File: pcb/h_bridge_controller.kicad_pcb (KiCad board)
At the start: 2 copper layers, 118.1 x 55.1 mm, 48 parts, among them P1 PWR_JACK_2.5x5.5, P2 HEADER_01X03_SMD_RA, P3 HEADER_01X03_SMD_RA, P4 HEADER_01X03_SMD_RA, P5 HEADER_01X03_SMD_RA, P6 HEADER_01X02_SMD_RA, P7 BNC_DOUBLE_RA, SW1 SPST_SLIDE_AS, T1 TERM_BLK_ANG_2_PIN, T2 TERM_BLK_ANG_2_PIN, T3 TERM_BLK_ANG_2_PIN, T4 TERM_BLK_ANG_2_PIN, T5 TERM_BLK_ANG_2_PIN, T6 TERM_BLK_ANG_2_PIN, T7 TERM_BLK_ANG_2_PIN, T8 TERM_BLK_ANG_2_PIN, U1 SSR_DC_6PIN, U2 SSR_DC_6PIN, U3 SSR_DC_6PIN, U4 SSR_DC_6PIN, U5 SSR_DC_6PIN, U6 SSR_DC_6PIN, U7 SSR_DC_6PIN, U8 SSR_DC_6PIN

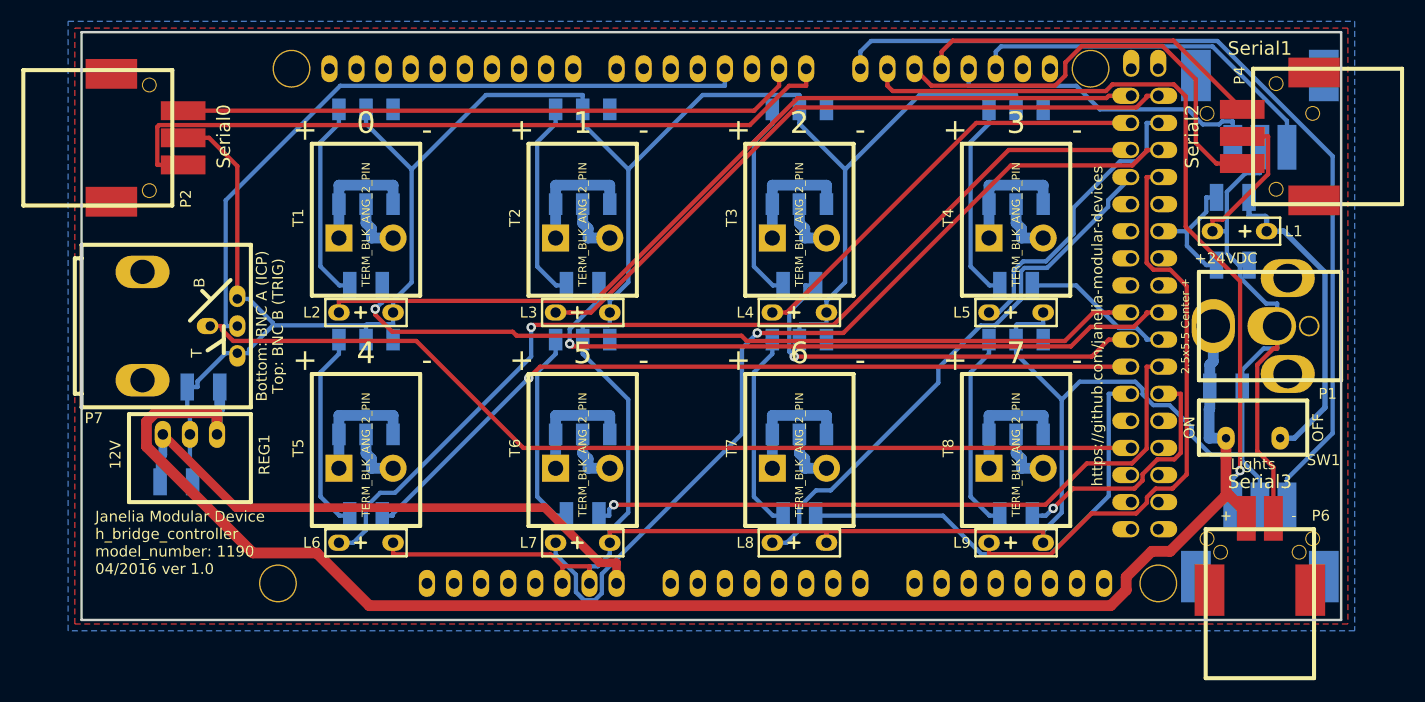
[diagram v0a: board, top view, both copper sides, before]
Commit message: Progress towards pcb1.0.
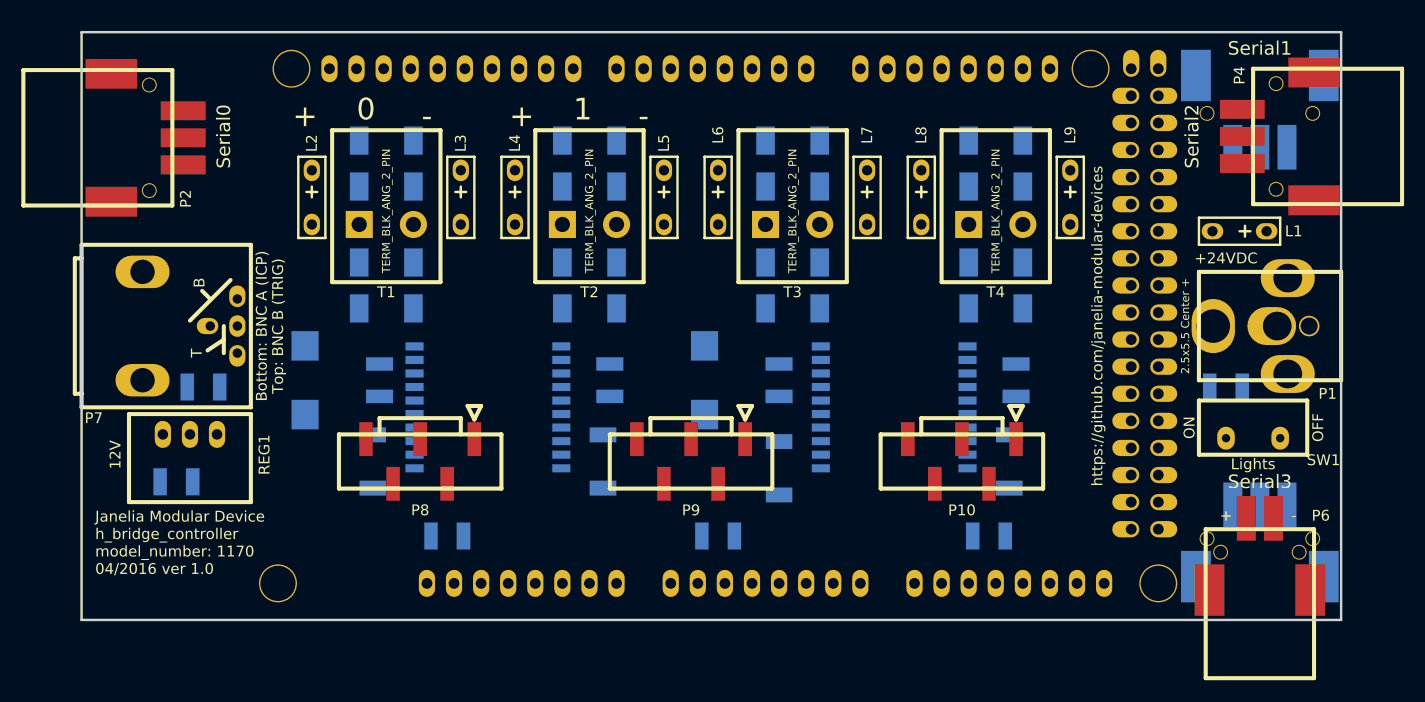
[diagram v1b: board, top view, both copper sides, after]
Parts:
- removed R10, R5, R6: 150, h_bridge_controller:SM1210
- removed T5, T6, T7, T8: TERM_BLK_ANG_2_PIN, h_bridge_controller:TERM_BLK_ANG_2_PIN
- removed U3, U4, U5, U6, U7, U8: SSR_DC_6PIN, h_bridge_controller:ASSR-1611
- added C4: 0.1uF, h_bridge_controller:SM1210, B.Cu at (121.3, 108.0)
- added C5: 0.1uF, h_bridge_controller:SM1210, B.Cu at (142.9, 108.0)
- added C6: 47uF, h_bridge_controller:SM2917_POL, B.Cu at (114.3, 108.0)
- added C7: 0.1uF, h_bridge_controller:SM1210, B.Cu at (158.8, 108.0)
- added C8: 0.1uF, h_bridge_controller:SM1210, B.Cu at (181.0, 108.0)
- added C9: 47uF, h_bridge_controller:SM2917_POL, B.Cu at (151.8, 108.0)
- added D1: diode_schottky_40V_1A, h_bridge_controller:DO-214AC(SMA), B.Cu at (119.4, 87.6)
- added D10: diode_schottky_40V_1A, h_bridge_controller:DO-214AC(SMA), B.Cu at (157.5, 99.1)
- added D11: diode_schottky_40V_1A, h_bridge_controller:DO-214AC(SMA), B.Cu at (162.6, 87.6)
- added D12: diode_schottky_40V_1A, h_bridge_controller:DO-214AC(SMA), B.Cu at (162.6, 99.1)
- added D13: diode_schottky_40V_1A, h_bridge_controller:DO-214AC(SMA), B.Cu at (176.5, 87.6)
- added D14: diode_schottky_40V_1A, h_bridge_controller:DO-214AC(SMA), B.Cu at (176.5, 99.1)
- added D15: diode_schottky_40V_1A, h_bridge_controller:DO-214AC(SMA), B.Cu at (181.6, 87.6)
- added D16: diode_schottky_40V_1A, h_bridge_controller:DO-214AC(SMA), B.Cu at (181.6, 99.1)
- added D2: diode_schottky_40V_1A, h_bridge_controller:DO-214AC(SMA), B.Cu at (119.4, 99.1)
- added D3: diode_schottky_40V_1A, h_bridge_controller:DO-214AC(SMA), B.Cu at (124.5, 87.6)
- added D4: diode_schottky_40V_1A, h_bridge_controller:DO-214AC(SMA), B.Cu at (124.5, 99.1)
- added D5: diode_schottky_40V_1A, h_bridge_controller:DO-214AC(SMA), B.Cu at (138.4, 87.6)
- added D6: diode_schottky_40V_1A, h_bridge_controller:DO-214AC(SMA), B.Cu at (138.4, 99.1)
- added D7: diode_schottky_40V_1A, h_bridge_controller:DO-214AC(SMA), B.Cu at (143.5, 87.6)
- added D8: diode_schottky_40V_1A, h_bridge_controller:DO-214AC(SMA), B.Cu at (143.5, 99.1)
- added D9: diode_schottky_40V_1A, h_bridge_controller:DO-214AC(SMA), B.Cu at (157.5, 87.6)
- added P10: HEADER_01X05_SMD_SHR, h_bridge_controller:Header_Shrouded_5_Pin_SMD, F.Cu at (175.9, 115.6)
- added P8: HEADER_01X05_SMD_SHR, h_bridge_controller:Header_Shrouded_5_Pin_SMD, F.Cu at (125.1, 115.6)
- added P9: HEADER_01X05_SMD_SHR, h_bridge_controller:Header_Shrouded_5_Pin_SMD, F.Cu at (150.5, 115.6)
- L2, L3, L4, L5, L6, L7, L8, L9: value LED_5V_GRN -> LED_24V
- R1: value 5.11k -> 0.5_2010; footprint h_bridge_controller:SM1210 -> h_bridge_controller:SM2010
- R2: value 1k -> 0.5_2010; footprint h_bridge_controller:SM1210 -> h_bridge_controller:SM2010
- R3, R4: value 150 -> 0.5_2010; footprint h_bridge_controller:SM1210 -> h_bridge_controller:SM2010
- R7, R8, R9: value 150 -> 180
- U1, U2: value SSR_DC_6PIN -> L298; footprint h_bridge_controller:ASSR-1611 -> h_bridge_controller:POWERSO20
- moved R1 84.4 mm to (120.7, 115.6), turned to 270 degrees
- moved R2 61.9 mm to (142.2, 115.6), turned to 270 degrees
- moved L6 46.3 mm to (153.0, 90.8), turned to 0 degrees
- moved R4 43.3 mm to (180.3, 115.6), turned to 270 degrees
- moved R3 42.4 mm to (158.8, 116.2), turned to 270 degrees
- moved L7 42.0 mm to (167.0, 90.8), turned to 0 degrees
- moved U2 37.5 mm to (169.5, 110.5), turned to 90 degrees
- moved L5 34.7 mm to (148.0, 90.8), turned to 0 degrees
- moved L8 34.3 mm to (172.1, 90.8), turned to 0 degrees
- moved L9 32.8 mm to (186.1, 90.8), turned to 0 degrees
- moved L4 28.8 mm to (134.0, 90.8), turned to 0 degrees
- moved U1 26.1 mm to (131.4, 110.5), turned to 90 degrees
- moved R9 17.9 mm to (178.4, 122.6), turned to 180 degrees
- moved L3 15.7 mm to (128.9, 90.8), turned to 0 degrees
- moved R8 12.8 mm to (153.0, 122.6), turned to 180 degrees
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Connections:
- ARDUINO1 pad 10: (no net) -> /PWM_2
- ARDUINO1 pad 11: (no net) -> /PWM_3
- ARDUINO1 pad 2: (no net) -> /SW_2
- ARDUINO1 pad 20: (no net) -> /SW_1
- ARDUINO1 pad 21: (no net) -> /SW_0
- ARDUINO1 pad 22: /LED_0 -> /DIR_0A
- ARDUINO1 pad 23: /LED_1 -> /DIR_0B
- ARDUINO1 pad 24: /LED_2 -> /DIR_1A
- ARDUINO1 pad 25: /LED_3 -> /DIR_1B
- ARDUINO1 pad 26: /LED_4 -> /DIR_2A
- ARDUINO1 pad 27: /LED_5 -> /DIR_2B
- ARDUINO1 pad 28: /LED_6 -> /DIR_3A
- ARDUINO1 pad 29: /LED_7 -> /DIR_3B
- ARDUINO1 pad 33: /LED_PWR_IN -> (no net)
- ARDUINO1 pad 38: /RELAY_0 -> (no net)
- ARDUINO1 pad 39: /RELAY_1 -> (no net)
- ARDUINO1 pad 40: /RELAY_2 -> (no net)
- ARDUINO1 pad 41: /RELAY_3 -> (no net)
- ARDUINO1 pad 42: /RELAY_4 -> (no net)
- ARDUINO1 pad 43: /RELAY_5 -> (no net)
- ARDUINO1 pad 44: /RELAY_6 -> (no net)
- ARDUINO1 pad 45: /RELAY_7 -> (no net)
- ARDUINO1 pad 5V_1: (no net) -> +5V
- ARDUINO1 pad 8: (no net) -> /PWM_0
- ARDUINO1 pad 9: (no net) -> /PWM_1
- ARDUINO1 pad A0: (no net) -> /SENSE_0
- ARDUINO1 pad A1: (no net) -> /SENSE_1
- ARDUINO1 pad A2: (no net) -> /SENSE_2
- ARDUINO1 pad A3: (no net) -> /SENSE_3
- L2 pad 1: /LED_0 -> /LED_PWR
- L2 pad 2: GND -> /OUT_0+
- L3 pad 1: /LED_1 -> /LED_PWR
- L3 pad 2: GND -> /OUT_0-
- L4 pad 1: /LED_2 -> /LED_PWR
- L4 pad 2: GND -> /OUT_1+
- L5 pad 1: /LED_3 -> /LED_PWR
- L5 pad 2: GND -> /OUT_1-
- L6 pad 1: /LED_4 -> /LED_PWR
- L6 pad 2: GND -> /OUT_2+
- L7 pad 1: /LED_5 -> /LED_PWR
- L7 pad 2: GND -> /OUT_2-
- L8 pad 1: /LED_6 -> /LED_PWR
- L8 pad 2: GND -> /OUT_3+
- L9 pad 1: /LED_7 -> /LED_PWR
- L9 pad 2: GND -> /OUT_3-
- R1 pad 1: /LED_PWR -> /SENSE_0
- R1 pad 2: /LED_PWR_IN -> GND
- R2 pad 1: /LED_PWR_IN -> /SENSE_1
- R3 pad 1: Net-(R3-Pad1) -> /SENSE_2
- R3 pad 2: /RELAY_0 -> GND
- R4 pad 1: Net-(R4-Pad1) -> /SENSE_3
- R4 pad 2: /RELAY_1 -> GND
- R7 pad 2: /RELAY_4 -> +5V
- R8 pad 2: /RELAY_5 -> +5V
- R9 pad 2: /RELAY_6 -> +5V
- U1 pad 1: Net-(R3-Pad1) -> GND
- U1 pad 2: GND -> /SENSE_0
- U1 pad 6: /OUT_0+ -> VAA
- U2 pad 1: Net-(R4-Pad1) -> GND
- U2 pad 2: GND -> /SENSE_2
- U2 pad 4: /OUT_1+ -> /OUT_2+
- U2 pad 5: /OUT_1- -> /OUT_2-
- U2 pad 6: /OUT_1+ -> VAA
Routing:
- net GND: track 410.8 -> 0.00 mm
- net VAA: track 149.0 -> 0.00 mm
- net /LED_4: track 92.4 -> 0.00 mm, vias 1 -> 0
- net /BNC_A: track 91.3 -> 0.00 mm
- net /TX3: track 85.2 -> 0.00 mm
- net /LED_5: track 83.6 -> 0.00 mm, vias 1 -> 0
- net /LED_0: track 83.4 -> 0.00 mm
- net /RELAY_4: track 76.1 -> 0.00 mm, vias 1 -> 0
- net /RELAY_0: track 76.1 -> 0.00 mm, vias 1 -> 0
- net /RX3: track 71.2 -> 0.00 mm, vias 1 -> 0
- net /RX0: track 70.0 -> 0.00 mm
- net /BNC_B: track 65.7 -> 0.00 mm
- net /LED_1: track 65.0 -> 0.00 mm
- net /RELAY_1: track 63.4 -> 0.00 mm, vias 1 -> 0
- net /RELAY_5: track 63.1 -> 0.00 mm, vias 1 -> 0
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- removed copper zone on B.Cu, net GND
- removed copper zone on F.Cu, net GND
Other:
- board text added: "Janelia Modular Device h_bridge_controller model_number: 1170 04/2016 ver 1.0"
- board text removed: "2"
- board text removed: "3"
- board text removed: "4"
- board text removed: "5"
- board text removed: "6"
- board text removed: "7"
- board text removed: "Janelia Modular Device h_bridge_controller model_number: 1190 04/2016 ver 1.0"
